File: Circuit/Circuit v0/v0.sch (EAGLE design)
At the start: 10 parts, among them U1 CD4051BE, U2 CD4051BE

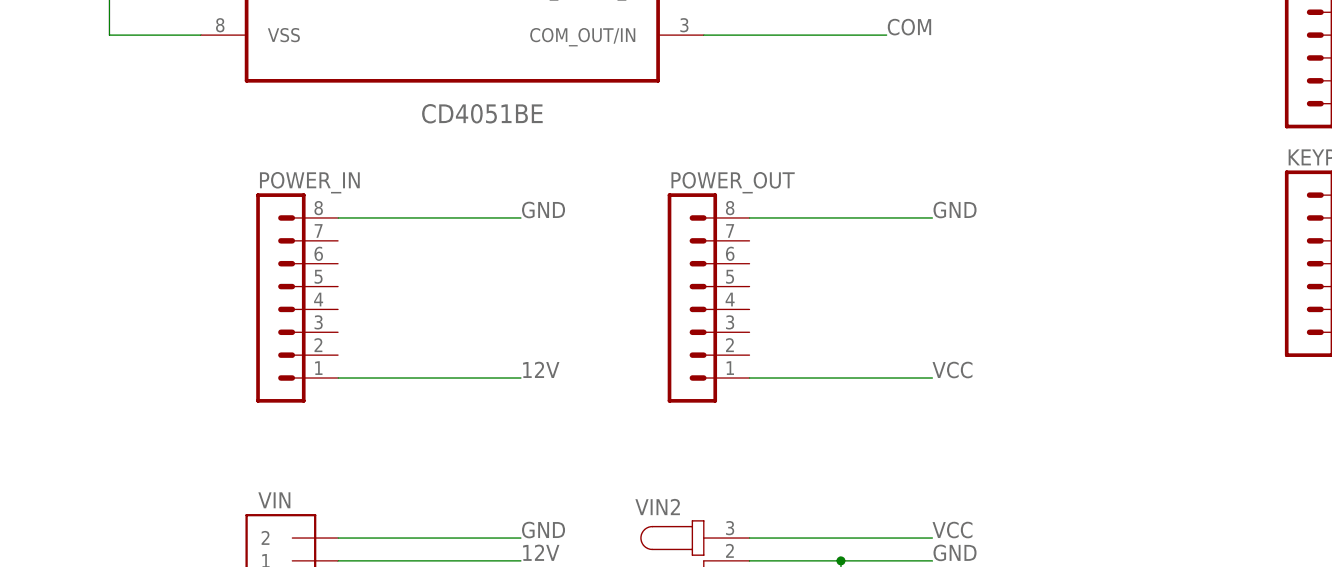
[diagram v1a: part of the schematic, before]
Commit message: circuit for fabrication
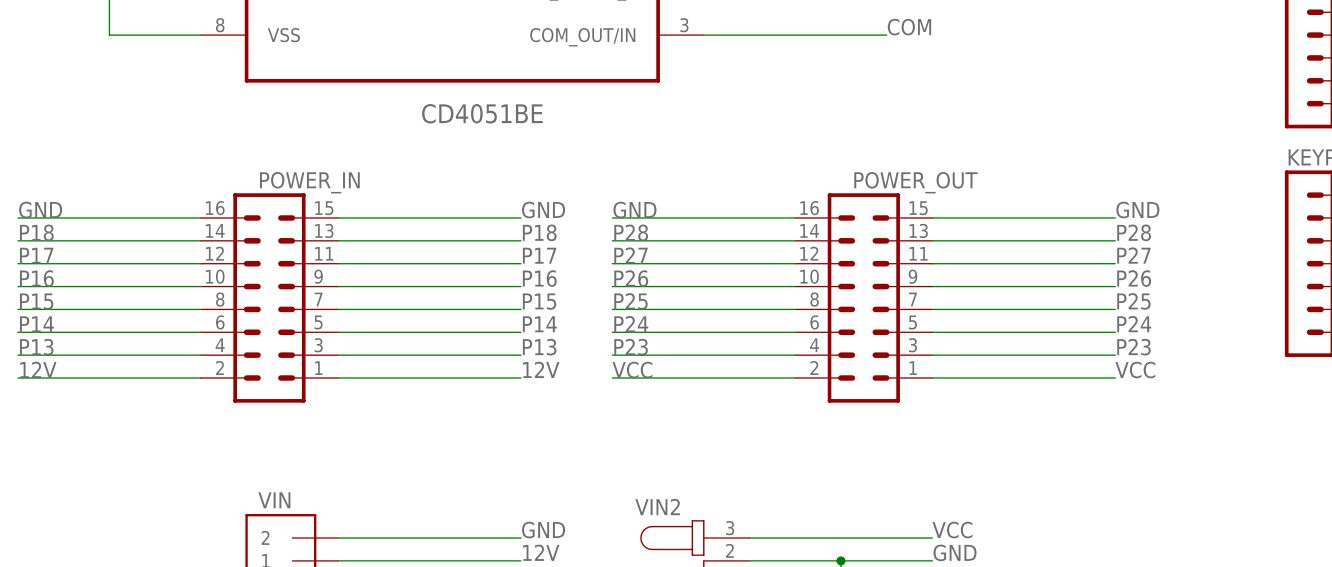
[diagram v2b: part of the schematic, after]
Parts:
- POWER_IN, POWER_OUT: device con-lstb:MA08-1 -> con-lstb:MA08-2
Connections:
- new net P13: POWER_IN.3, POWER_IN.4
- new net P14: POWER_IN.5, POWER_IN.6
- new net P15: POWER_IN.7, POWER_IN.8
- new net P16: POWER_IN.10, POWER_IN.9
- new net P17: POWER_IN.11, POWER_IN.12
- new net P18: POWER_IN.13, POWER_IN.14
- new net P23: POWER_OUT.3, POWER_OUT.4
- new net P24: POWER_OUT.5, POWER_OUT.6
- new net P25: POWER_OUT.7, POWER_OUT.8
- new net P26: POWER_OUT.10, POWER_OUT.9
- new net P27: POWER_OUT.11, POWER_OUT.12
- new net P28: POWER_OUT.13, POWER_OUT.14
- net 12V: now also POWER_IN.2
- net GND: now also POWER_IN.15, POWER_IN.16, POWER_OUT.15, POWER_OUT.16; no longer POWER_IN.8, POWER_OUT.8
- net VCC: now also POWER_OUT.2
